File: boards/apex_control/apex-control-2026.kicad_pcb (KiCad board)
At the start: 4 copper layers, 50 x 100 mm, 18 parts, among them J1 UJ20-C-H-G-SMT-5-P16, U1 ADXL375, U10 MKL26Z128VFM4, U11 W25Q64JW, U12 MAYA-W166-00B, U2 MMC5983MA, U3 ICM-45686, U4 BMP581, U5 RTMC-G2-4IQ48, U6 MIMXRT1171DVMAB, U7 TPS62086, U8 TPS62825, U9 LM66200, Y1 Crystal_GND24

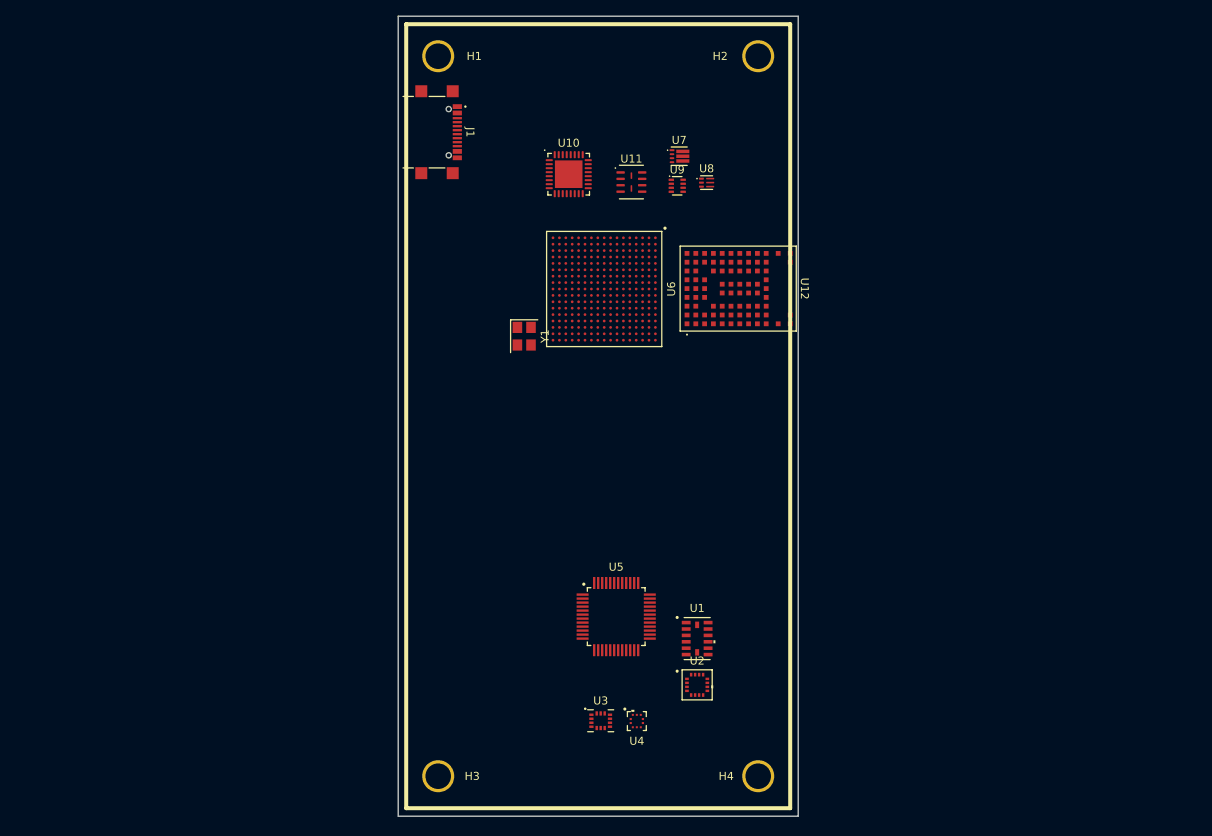
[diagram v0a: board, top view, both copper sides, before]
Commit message: More placement
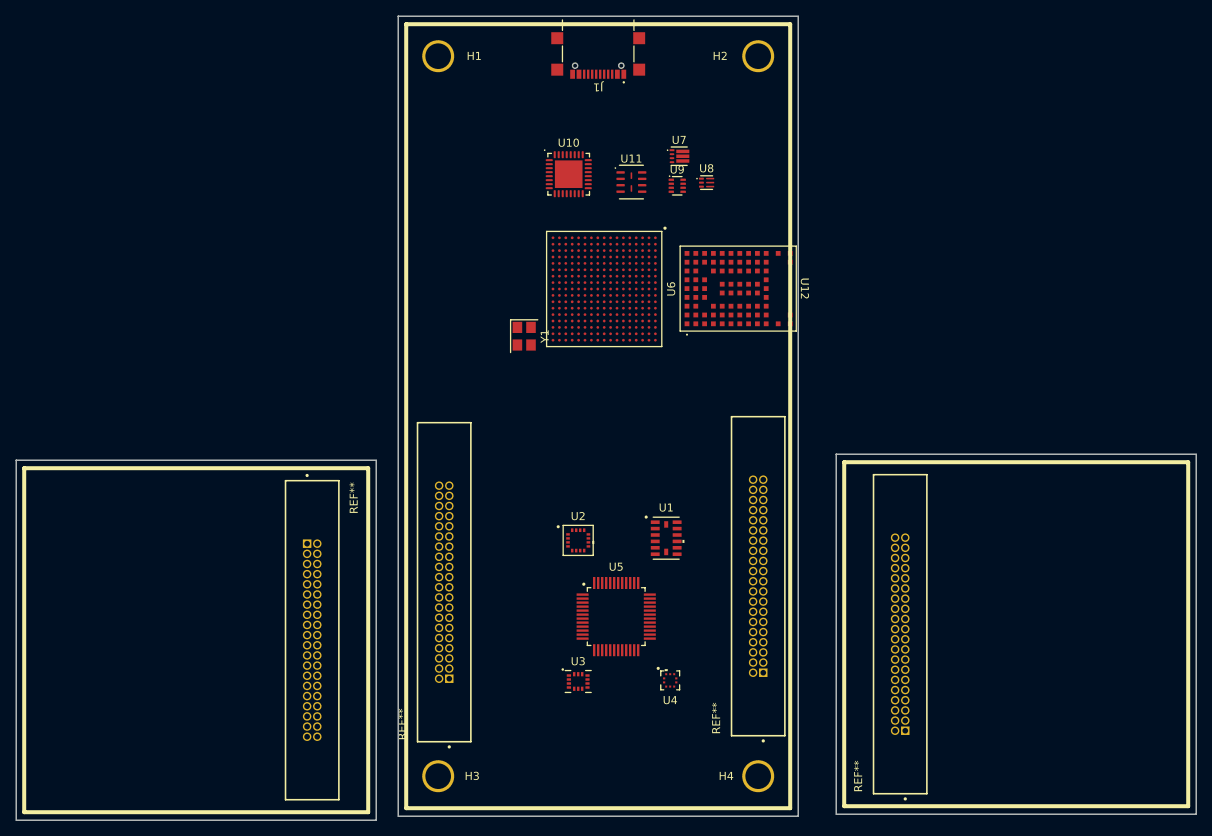
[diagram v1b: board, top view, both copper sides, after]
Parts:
- added REF**: SAMTEC_EHF-120-01-L-D, APEX_FOOTPRINTS:SAMTEC_EHF-120-01-L-D, F.Cu at (137.8, 127.2)
- added REF**: SAMTEC_EHF-120-01-L-D, APEX_FOOTPRINTS:SAMTEC_EHF-120-01-L-D, F.Cu at (120.0, 120.0)
- added REF**: SAMTEC_EHF-120-01-L-D, APEX_FOOTPRINTS:SAMTEC_EHF-120-01-L-D, F.Cu at (80.8, 120.8)
- added REF**: SAMTEC_EHF-120-01-L-D, APEX_FOOTPRINTS:SAMTEC_EHF-120-01-L-D, F.Cu at (64.2, 128.0)
- moved J1 23.5 mm to (100.0, 53.9), turned to 180 degrees
- moved U2 23.4 mm to (97.5, 115.5)
- moved U1 13.1 mm to (108.5, 115.2)
- moved U4 6.58 mm to (109.0, 133.0)
- moved U3 5.65 mm to (97.5, 133.2)
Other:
- board size 50 x 100 mm -> 147.5 x 100.5 mm

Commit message: Worked on stuff
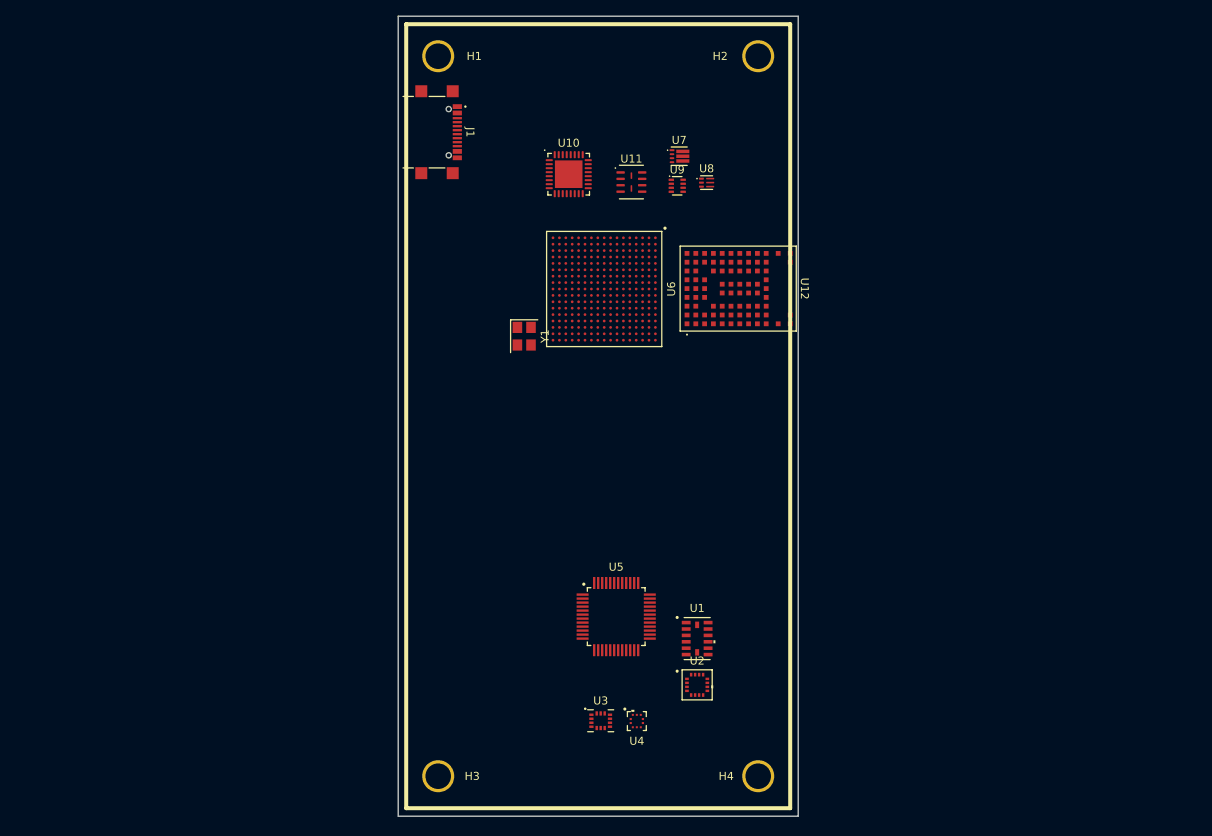
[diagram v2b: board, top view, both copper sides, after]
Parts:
- removed REF** (x4): SAMTEC_EHF-120-01-L-D, APEX_FOOTPRINTS:SAMTEC_EHF-120-01-L-D
- moved J1 23.5 mm to (79.0, 64.5), turned to -90 degrees
- moved U2 23.4 mm to (112.4, 133.6)
- moved U1 13.1 mm to (112.4, 127.8)
- moved U4 6.58 mm to (104.8, 138.1)
- moved U3 5.65 mm to (100.3, 138.1)
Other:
- board size 147.5 x 100.5 mm -> 50 x 100 mm
